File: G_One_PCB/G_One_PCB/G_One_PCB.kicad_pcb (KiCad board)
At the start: 2 copper layers, 91 parts, among them K01(ESC)1 KEYSW, K02(F1)1 KEYSW, K03(F2)1 KEYSW, K04(F3)1 KEYSW, K05(F4)1 KEYSW, K07(F5)1 KEYSW, K10(M0)1 KEYSW, K11(_`_)1 KEYSW, K12(1!)1 KEYSW, K13(2@)1 KEYSW, K14(3#)1 KEYSW, K15(4$)1 KEYSW, K16(5%)1 KEYSW, K17(6^)1 KEYSW, K20(M1)1 KEYSW, K21(Tap)1 KEYSW, K22(Q)1 KEYSW, K23(W)1 KEYSW, K24(E)1 KEYSW, K25(R)1 KEYSW, K26(T)1 KEYSW, K27(P)1 KEYSW, K28(IoT0)1 KEYSW, K30(M2)1 KEYSW, K31(Caps_Lock)1 KEYSW, K32(A)1 KEYSW, K33(S)1 KEYSW, K34(D)1 KEYSW, K35(F)1 KEYSW, K36(G)1 KEYSW, K37(H)1 KEYSW, K38(IoT1)1 KEYSW, K40(M3)1 KEYSW, K41(L_Shift)1 KEYSW, K42(Z)1 KEYSW, K43(X)1 KEYSW, K44(C)1 KEYSW, K45(V)1 KEYSW, K46(B)1 KEYSW, K48(IoT2)1 KEYSW, K50(M4)1 KEYSW, K51(L_CTRL)1 KEYSW, K52(Win)1 KEYSW, K53(L_ALT)1 KEYSW, K54(Space)1 KEYSW

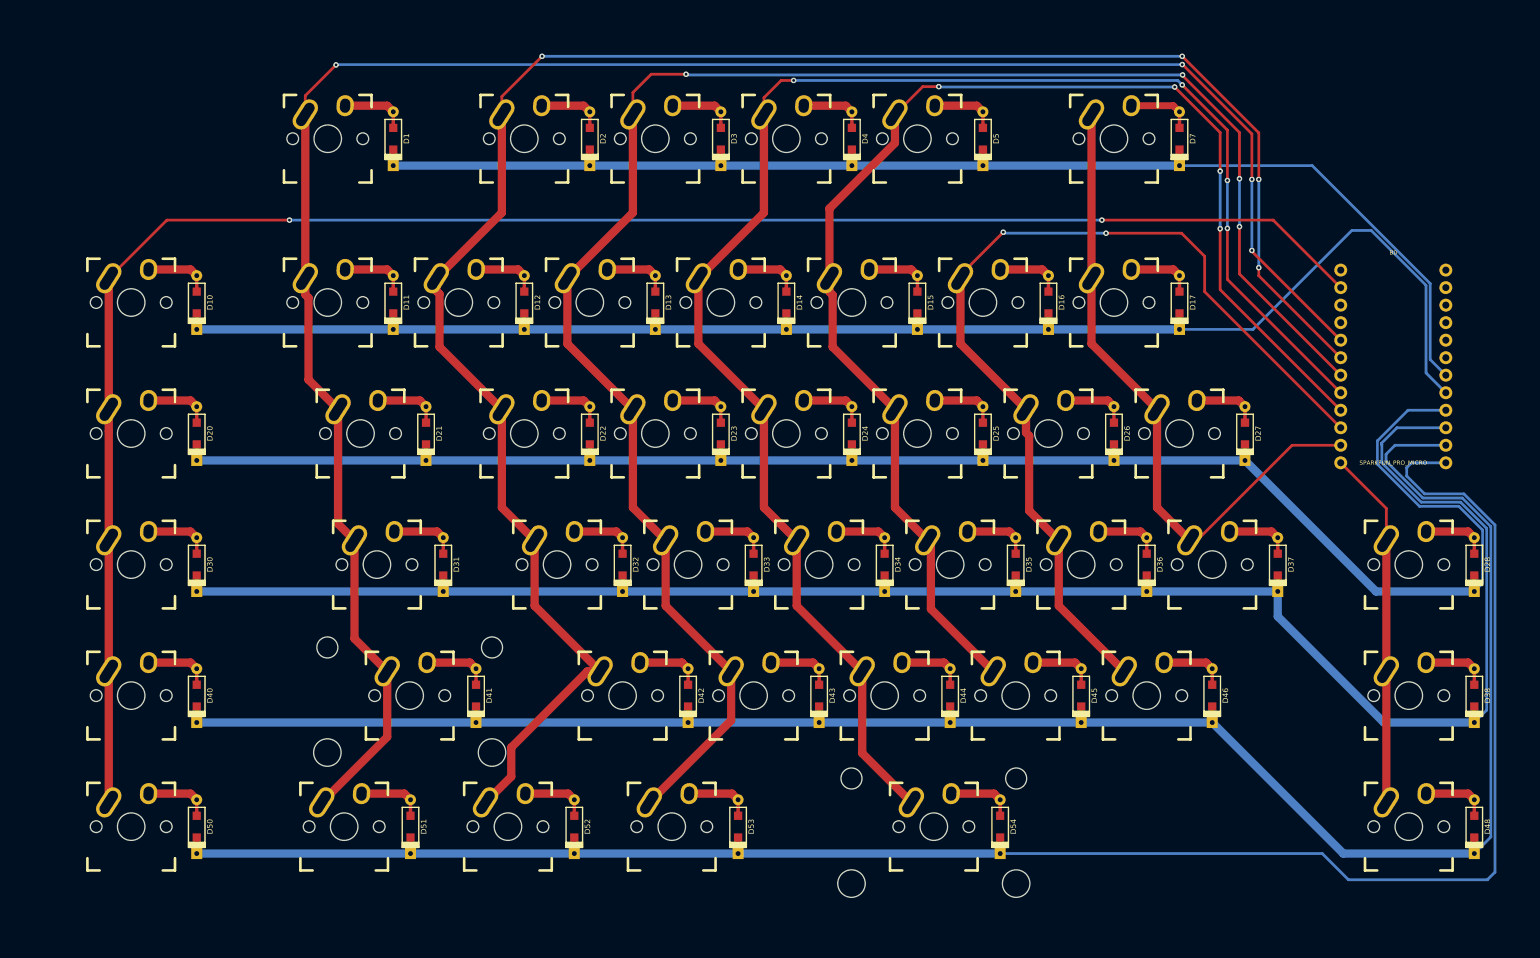
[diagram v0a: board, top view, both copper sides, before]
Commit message: pcb 수정
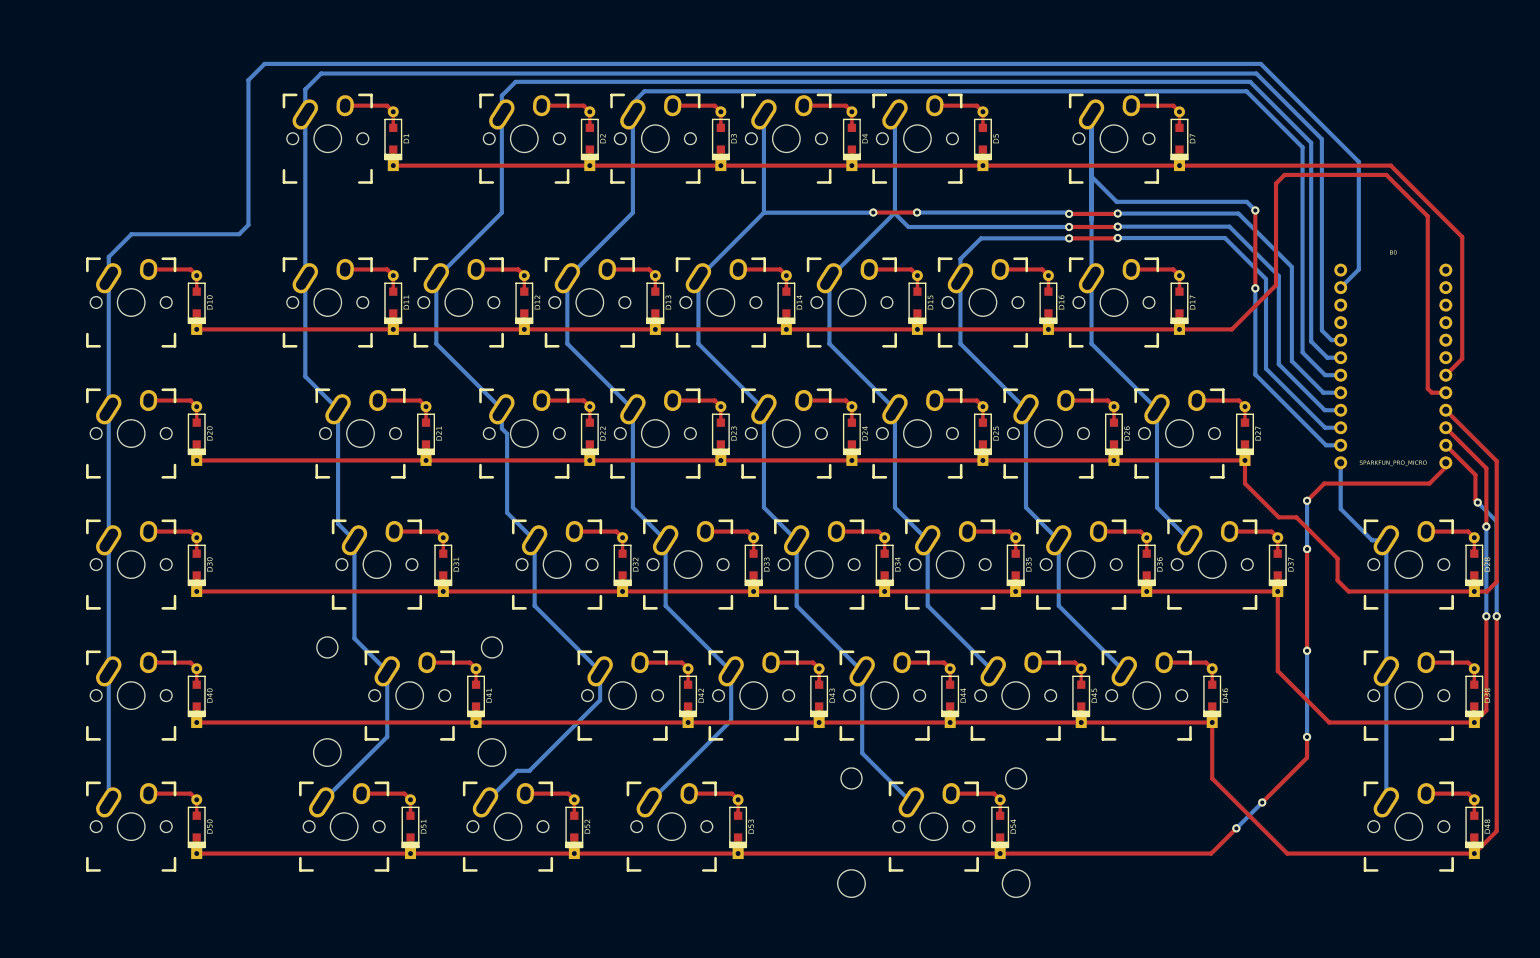
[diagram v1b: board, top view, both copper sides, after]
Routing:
- net /col7: track 95.2 -> 158.2 mm, vias 0 -> 2
- net /col0: track 262.2 -> 309.4 mm, vias 2 -> 0
- net /row5: track 263.5 -> 226.8 mm, vias 0 -> 6
- net /row1: track 204.3 -> 226.6 mm
- net /col4: track 235.0 -> 219.0 mm
- net /col5: track 193.6 -> 178.6 mm, vias 4 -> 2
- net /row3: track 256.4 -> 245.8 mm, vias 0 -> 2
- net /row4: track 270.9 -> 261.5 mm, vias 0 -> 2
- net /row0: track 171.7 -> 180.3 mm
- net /row2: track 236.9 -> 228.7 mm
- net /col1: track 289.9 -> 295.6 mm, vias 4 -> 0
- net /col6: track 140.3 -> 145.0 mm
- net /col3: track 255.5 -> 257.9 mm, vias 4 -> 0
- net /col2: track 278.4 -> 280.1 mm, vias 4 -> 0
- net /col8: track 52.0 -> 53.2 mm

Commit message: PCB 제작 완료 및 거버 파일 생성
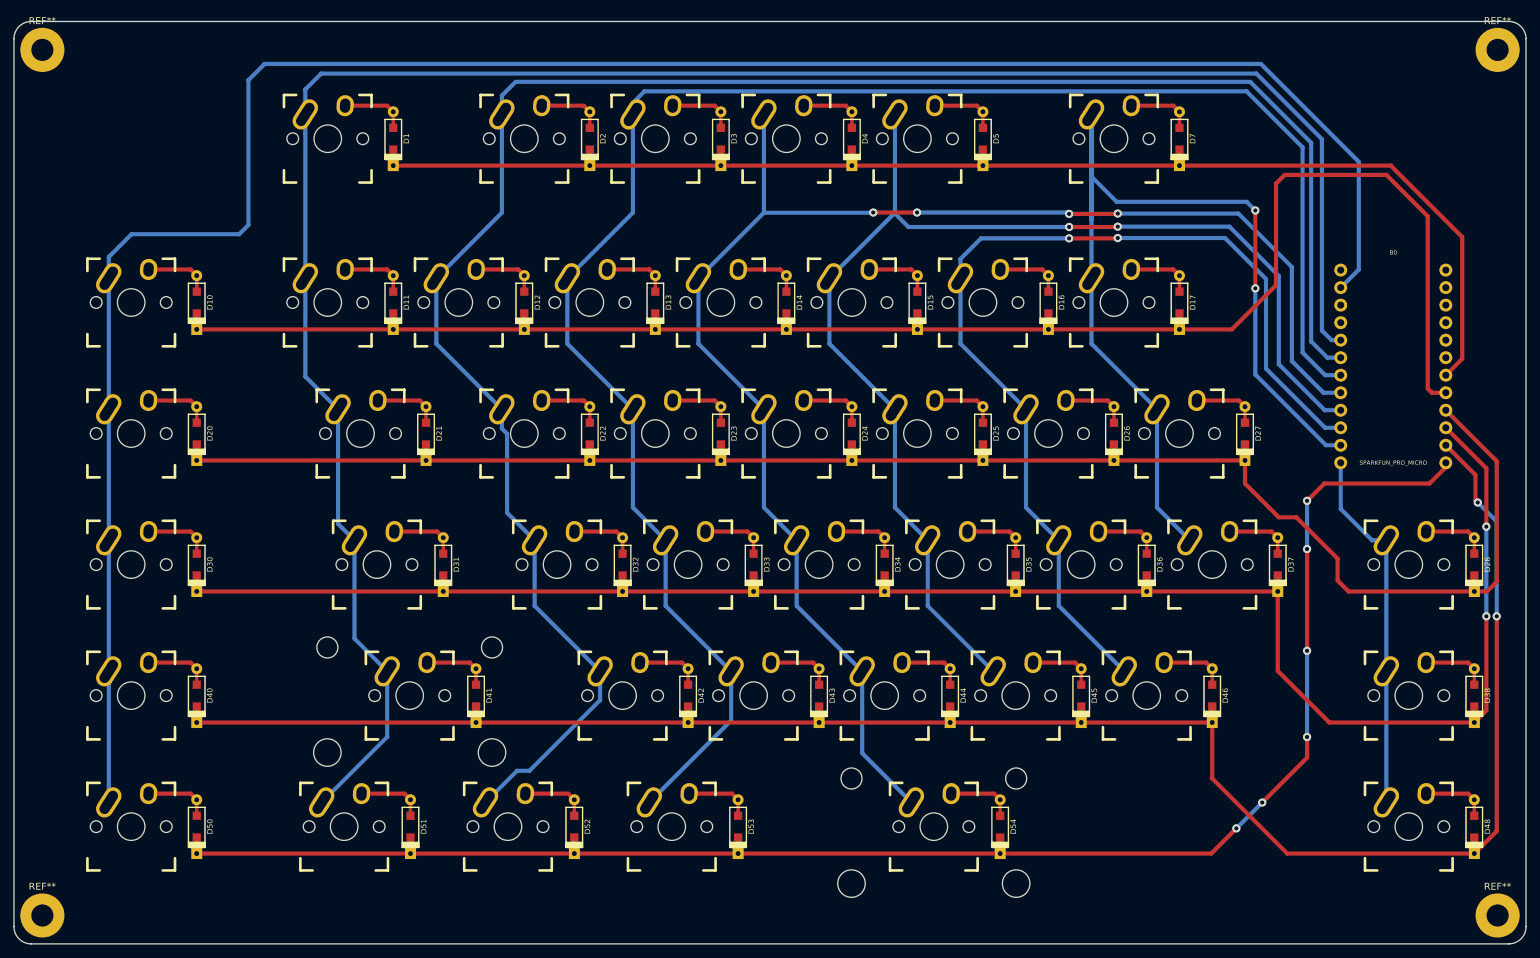
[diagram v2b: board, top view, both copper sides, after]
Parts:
- added REF**: MountingHole_3.2mm_M3_Pad, MountingHole:MountingHole_3.2mm_M3_Pad, F.Cu at (215.1, -4.12)
- added REF**: MountingHole_3.2mm_M3_Pad, MountingHole:MountingHole_3.2mm_M3_Pad, F.Cu at (215.1, -129.6)
- added REF**: MountingHole_3.2mm_M3_Pad, MountingHole:MountingHole_3.2mm_M3_Pad, F.Cu at (4.12, -4.12)
- added REF**: MountingHole_3.2mm_M3_Pad, MountingHole:MountingHole_3.2mm_M3_Pad, F.Cu at (4.12, -129.6)
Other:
- board outline added: 219.2 x 133.8 mm
